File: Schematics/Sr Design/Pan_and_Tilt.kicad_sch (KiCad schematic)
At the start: 3 parts, among them J2 Raspberry_Pi_4, M1 Motor_Servo, M2 Motor_Servo

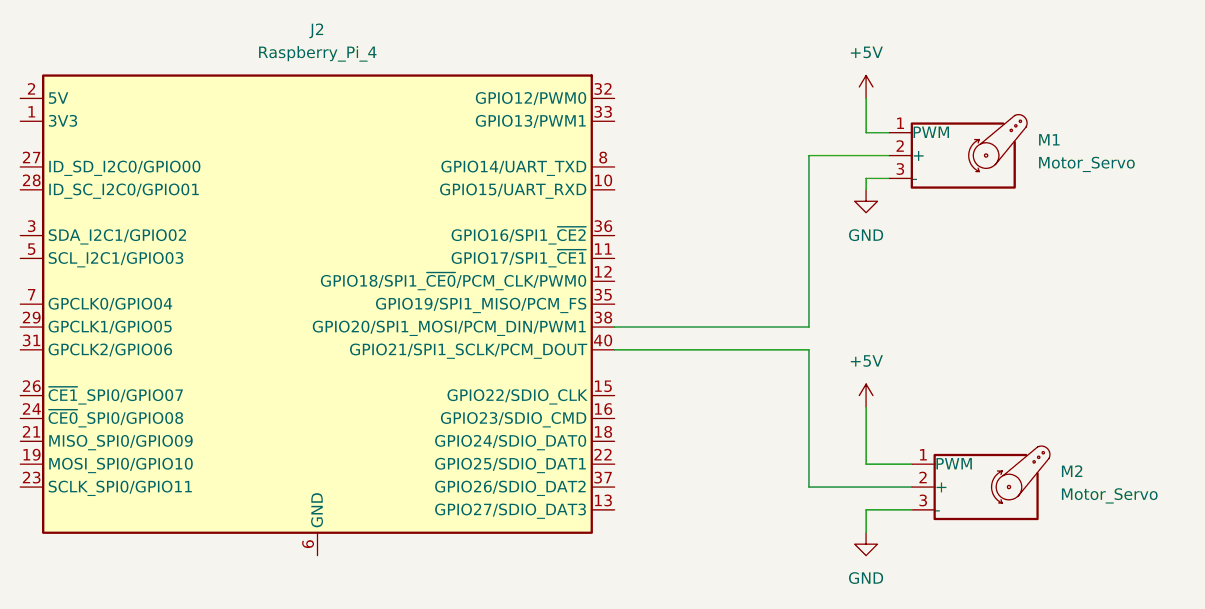
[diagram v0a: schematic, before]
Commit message: scematics update
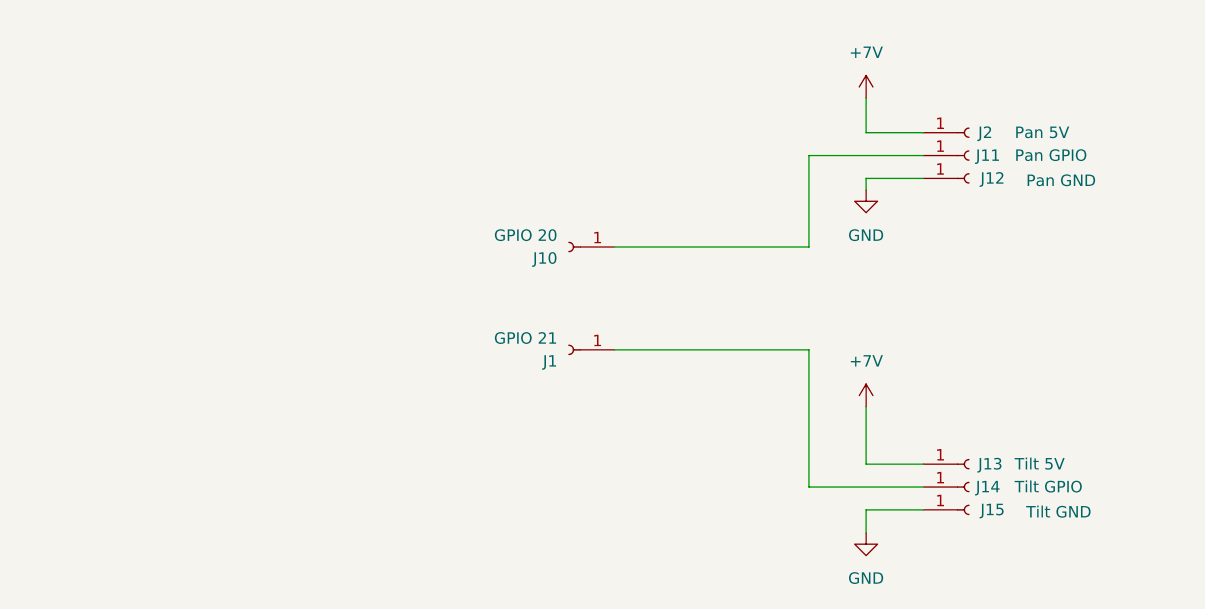
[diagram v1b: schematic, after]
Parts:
- removed J2: Raspberry_Pi_4, symbol Connector:Raspberry_Pi_4
- removed M1, M2: Motor_Servo, symbol Motor:Motor_Servo
- added J1: GPIO 21, Connector_PinHeader_1.00mm:PinHeader_1x01_P1.00mm_Vertical, symbol Connector:Conn_01x01_Socket
- added J10: GPIO 20, Connector_PinHeader_1.00mm:PinHeader_1x01_P1.00mm_Vertical, symbol Connector:Conn_01x01_Socket
- added J11: Pan GPIO, Connector_PinHeader_1.00mm:PinHeader_1x01_P1.00mm_Vertical, symbol Connector:Conn_01x01_Socket
- added J12: Pan GND, Connector_PinHeader_1.00mm:PinHeader_1x01_P1.00mm_Vertical, symbol Connector:Conn_01x01_Socket
- added J13: Tilt 5V, Connector_PinHeader_1.00mm:PinHeader_1x01_P1.00mm_Vertical, symbol Connector:Conn_01x01_Socket
- added J14: Tilt GPIO, Connector_PinHeader_1.00mm:PinHeader_1x01_P1.00mm_Vertical, symbol Connector:Conn_01x01_Socket
- added J15: Tilt GND, Connector_PinHeader_1.00mm:PinHeader_1x01_P1.00mm_Vertical, symbol Connector:Conn_01x01_Socket
- added J2: Pan 5V, Connector_PinHeader_1.00mm:PinHeader_1x01_P1.00mm_Vertical, symbol Connector:Conn_01x01_Socket
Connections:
- net GND: now also J12.1 (Pin_1), J15.1 (Pin_1)
- new net: J10.1 (Pin_1), J11.1 (Pin_1)
- new net: J1.1 (Pin_1), J14.1 (Pin_1)
- new net +7V: J13.1 (Pin_1), J2.1 (Pin_1)
